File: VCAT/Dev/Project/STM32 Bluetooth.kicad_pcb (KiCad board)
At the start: 4 copper layers, 56 x 47.5 mm, 41 parts, among them J1 USB_C_Receptacle_USB2.0, J2 Conn_01x04, J3 TC2030, J4 Conn_Coaxial, SW1 SW_Push, U1 MIC5365-3.3YD5, U2 USBLC6-2SC6, U3 STM32WB55CEU, X1 32kHz768, X2 32MHz

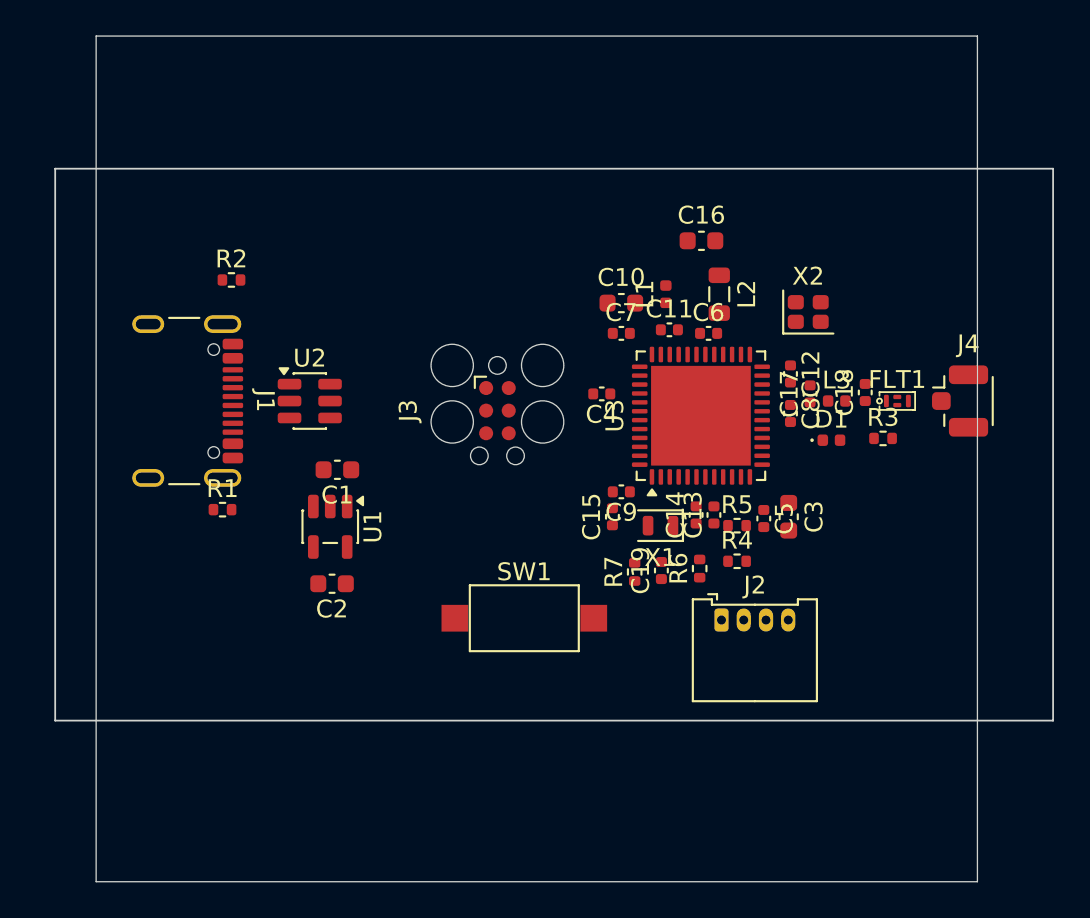
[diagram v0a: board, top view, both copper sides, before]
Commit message: final
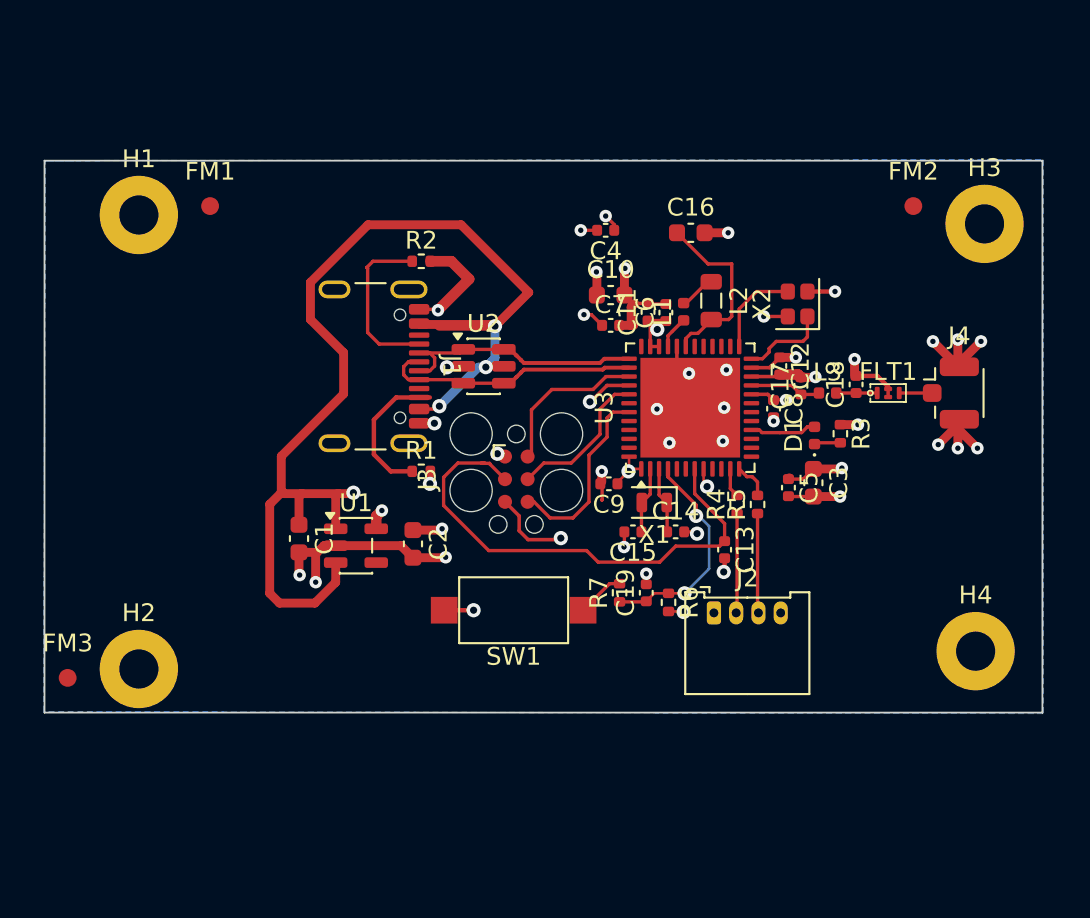
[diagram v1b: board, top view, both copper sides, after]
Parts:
- added FM1: Fiducial, Fiducial:Fiducial_1mm_Mask2mm, F.Cu at (73.4, 69.0)
- added FM2: Fiducial, Fiducial:Fiducial_1mm_Mask2mm, F.Cu at (112.9, 69.0)
- added FM3: Fiducial, Fiducial:Fiducial_1mm_Mask2mm, F.Cu at (65.4, 95.5)
- added H1: MountingHole_Pad, MountingHole:MountingHole_2.2mm_M2_Pad, F.Cu at (69.4, 69.5)
- added H2: MountingHole_Pad, MountingHole:MountingHole_2.2mm_M2_Pad, F.Cu at (69.4, 95.0)
- added H3: MountingHole_Pad, MountingHole:MountingHole_2.2mm_M2_Pad, F.Cu at (116.9, 70.0)
- added H4: MountingHole_Pad, MountingHole:MountingHole_2.2mm_M2_Pad, F.Cu at (116.4, 94.0)
- moved R1 11.4 mm to (85.3, 84.0)
- moved R2 10.7 mm to (85.3, 72.2)
- moved J1 10.6 mm to (81.5, 78.0)
- moved U2 9.96 mm to (88.8, 78.0)
- moved C4 9.19 mm to (95.6, 70.4)
- moved C2 5.06 mm to (84.8, 88.0), turned to -90 degrees
- moved C1 4.42 mm to (78.4, 87.7), turned to -90 degrees
- moved J3 3.99 mm to (90.6, 84.4)
- moved R4 3.19 mm to (103.0, 85.8), turned to 90 degrees
- moved C6 2.67 mm to (99.0, 75.0), turned to 90 degrees
- moved R6 2.58 mm to (99.2, 91.3), turned to -90 degrees
- moved R3 2.41 mm to (108.8, 81.8), turned to -90 degrees
- moved C3 2.36 mm to (107.3, 84.6)
- moved C5 2.22 mm to (105.9, 84.9)
- moved C13 2.04 mm to (102.3, 88.3), turned to -90 degrees
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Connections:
- J1 pad A6: Net-(J1-D+-PadA6) -> /USB_D+
- J1 pad A7: Net-(J1-D--PadA7) -> /USB_D-
- J1 pad B6: Net-(J1-D+-PadA6) -> /USB_D+
- J1 pad B7: Net-(J1-D--PadA7) -> /USB_D-
- U2 pad 1: Net-(J1-D--PadA7) -> /USB_D-
- U2 pad 3: Net-(J1-D+-PadA6) -> /USB_D+
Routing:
- net GND: track 0.00 -> 86.9 mm, vias 0 -> 36
- net +5V: track 0.00 -> 67.2 mm, vias 0 -> 4
- net /SWD_NRST: track 0.00 -> 28.3 mm
- net +3V3: track 0.00 -> 27.3 mm, vias 0 -> 14
- net /USB_D-: track 0.00 -> 14.7 mm
- net /USB_D+: track 0.00 -> 14.7 mm
- net /BOOT0: track 0.00 -> 12.9 mm, vias 0 -> 2
- net /SWD_TRC: track 0.00 -> 10.7 mm
- net /SMPSFB: track 0.00 -> 10.3 mm
- net Net-(J1-CC1): track 0.00 -> 9.53 mm
- net /SWD_DIO: track 0.00 -> 8.97 mm
- net /SWD_CLK: track 0.00 -> 8.50 mm
- net Net-(J1-CC2): track 0.00 -> 8.16 mm
- net /UART_TXC: track 0.00 -> 5.60 mm
- net /UART_RXC: track 0.00 -> 5.60 mm
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- added copper zone on B.Cu, net (none)
- added copper zone on In2.Cu, net +3V3
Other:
- board size 56 x 47.5 mm -> 56.1 x 31 mm
